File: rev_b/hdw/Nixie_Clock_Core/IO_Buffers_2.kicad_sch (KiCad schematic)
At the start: 10 parts

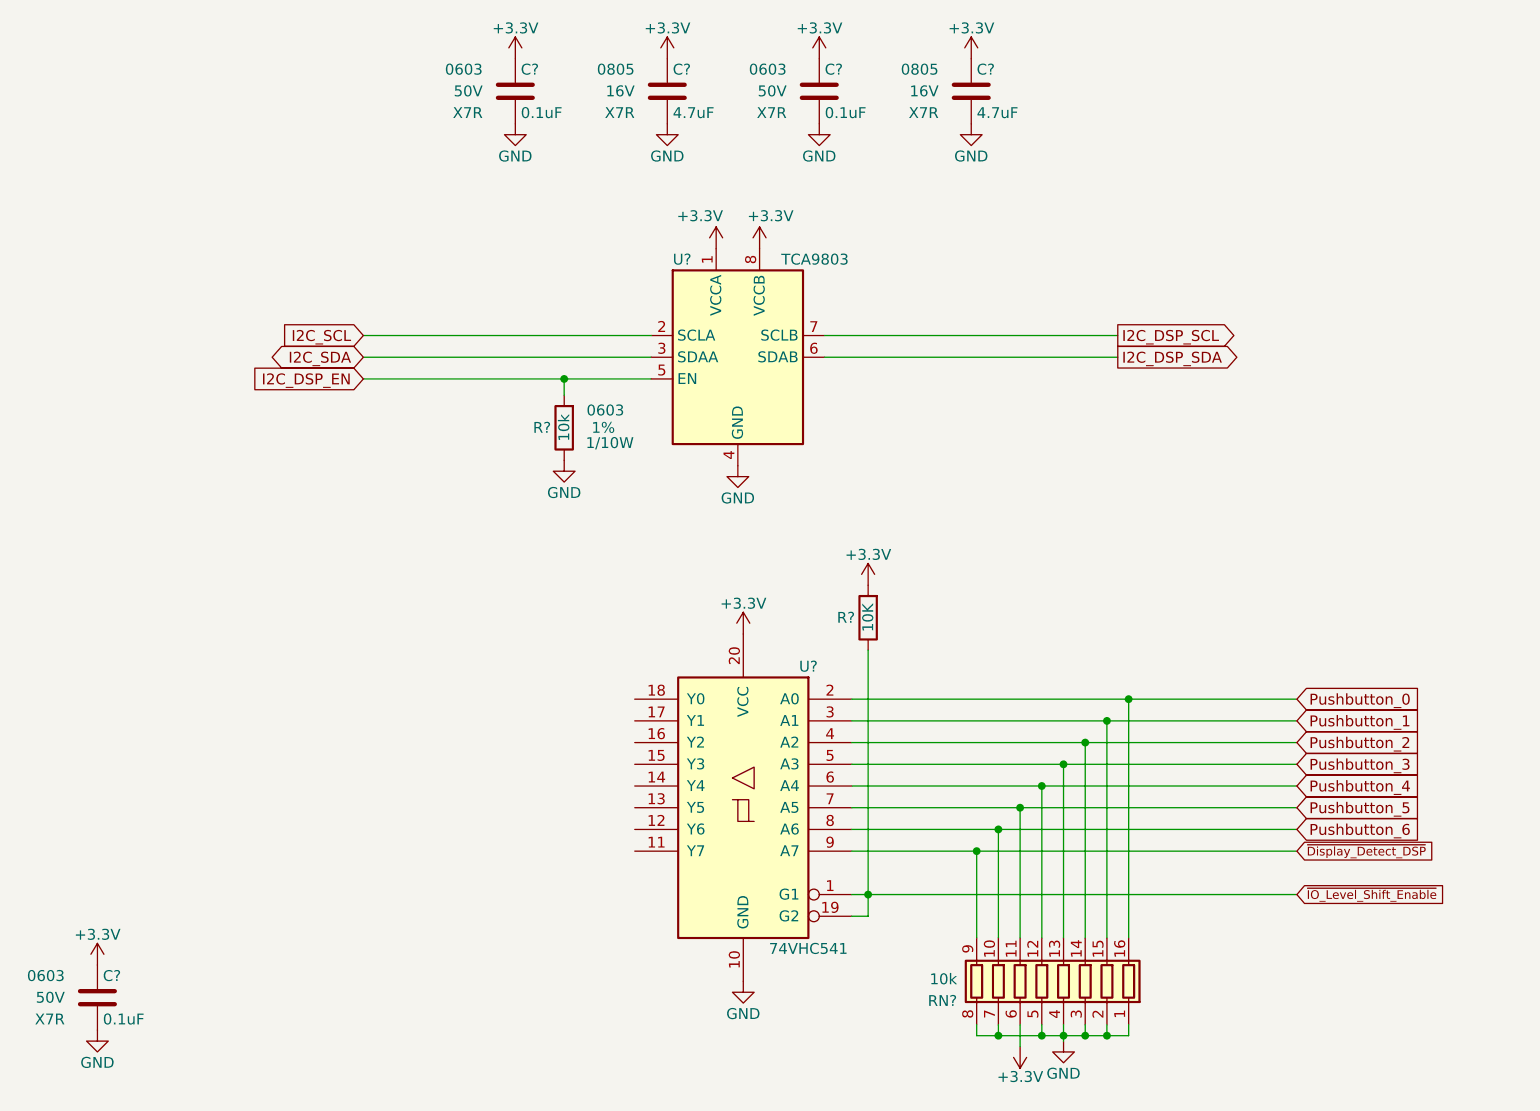
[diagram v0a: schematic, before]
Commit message: more rev b sch progress
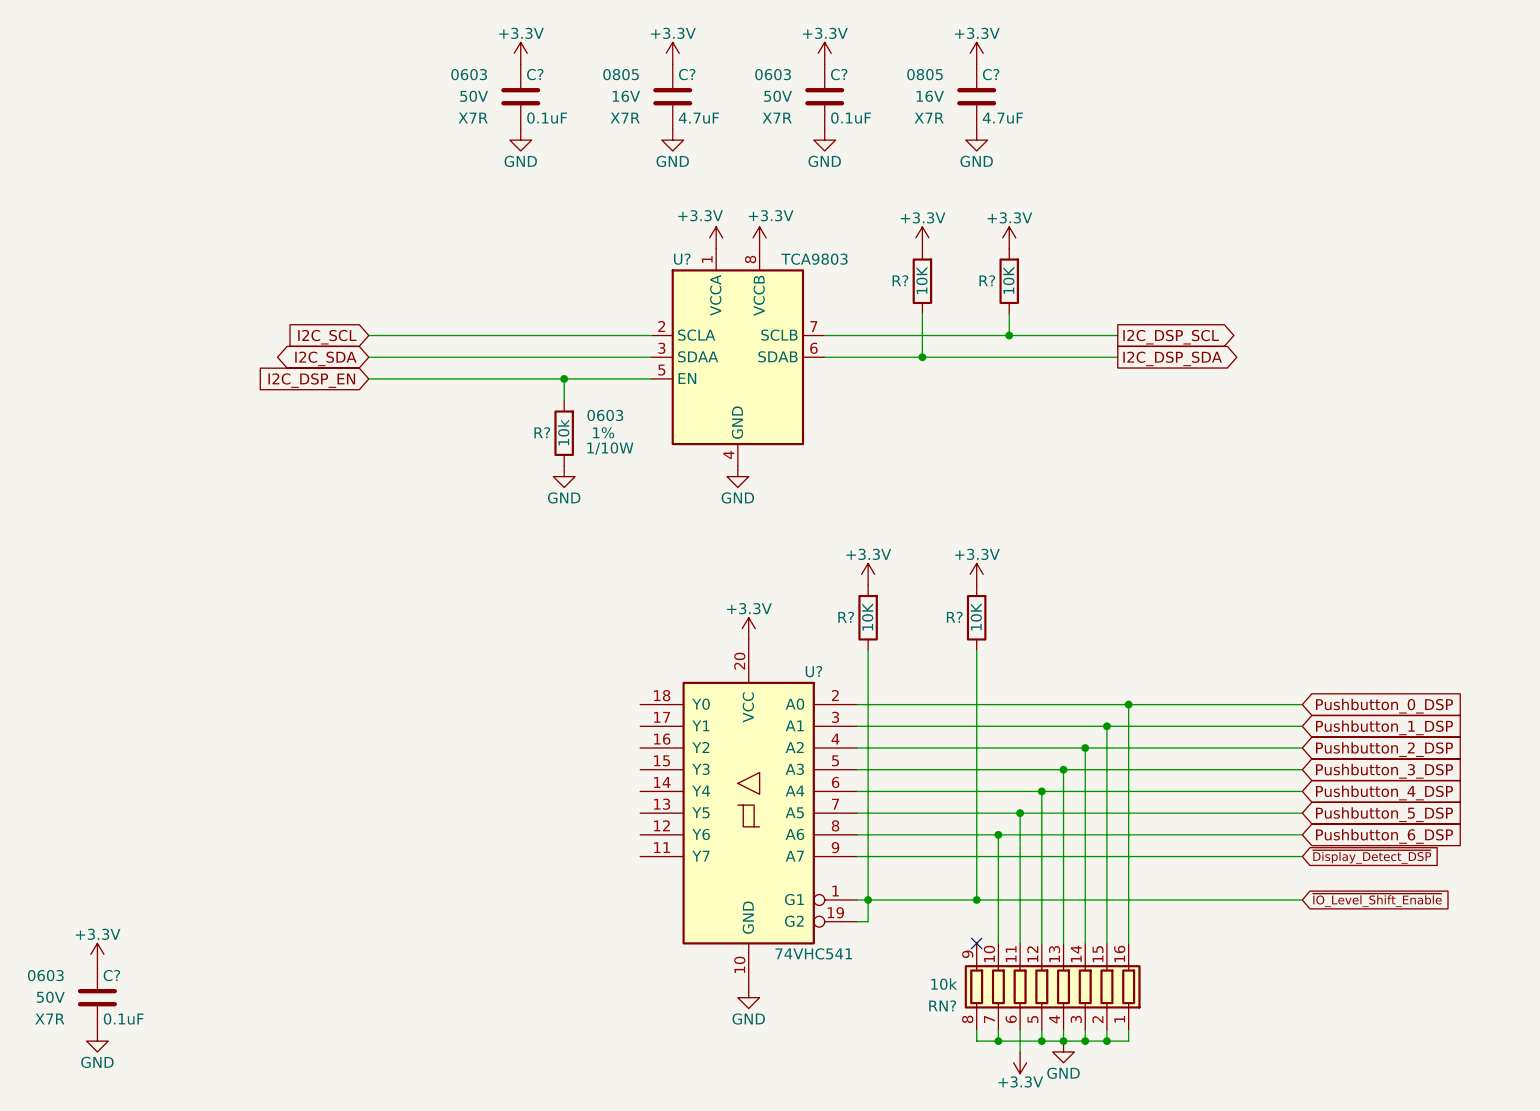
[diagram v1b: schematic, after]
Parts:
- added R? (x3): 10K, Resistors_SMD:R_0603, symbol Custom_Library:R_Custom
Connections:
- net +3.3V: now also R?.1, R?.1, R?.1
- net I2C_DSP_SCL: now also R?.2
- net I2C_DSP_SDA: now also R?.2
- net ~{Display_Detect_DSP}: no longer RN?.9 (R8.2)
- net ~{IO_Level_Shift_Enable}: now also R?.2
- net Pushbutton_0 renamed Pushbutton_0_DSP
- net Pushbutton_1 renamed Pushbutton_1_DSP
- net Pushbutton_2 renamed Pushbutton_2_DSP
- net Pushbutton_3 renamed Pushbutton_3_DSP
- net Pushbutton_4 renamed Pushbutton_4_DSP
- net Pushbutton_5 renamed Pushbutton_5_DSP
- net Pushbutton_6 renamed Pushbutton_6_DSP
- no-connect marks 0 -> 1
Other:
- moved on the sheet: C?, R?, RN?, U?

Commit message: more carrier board progress
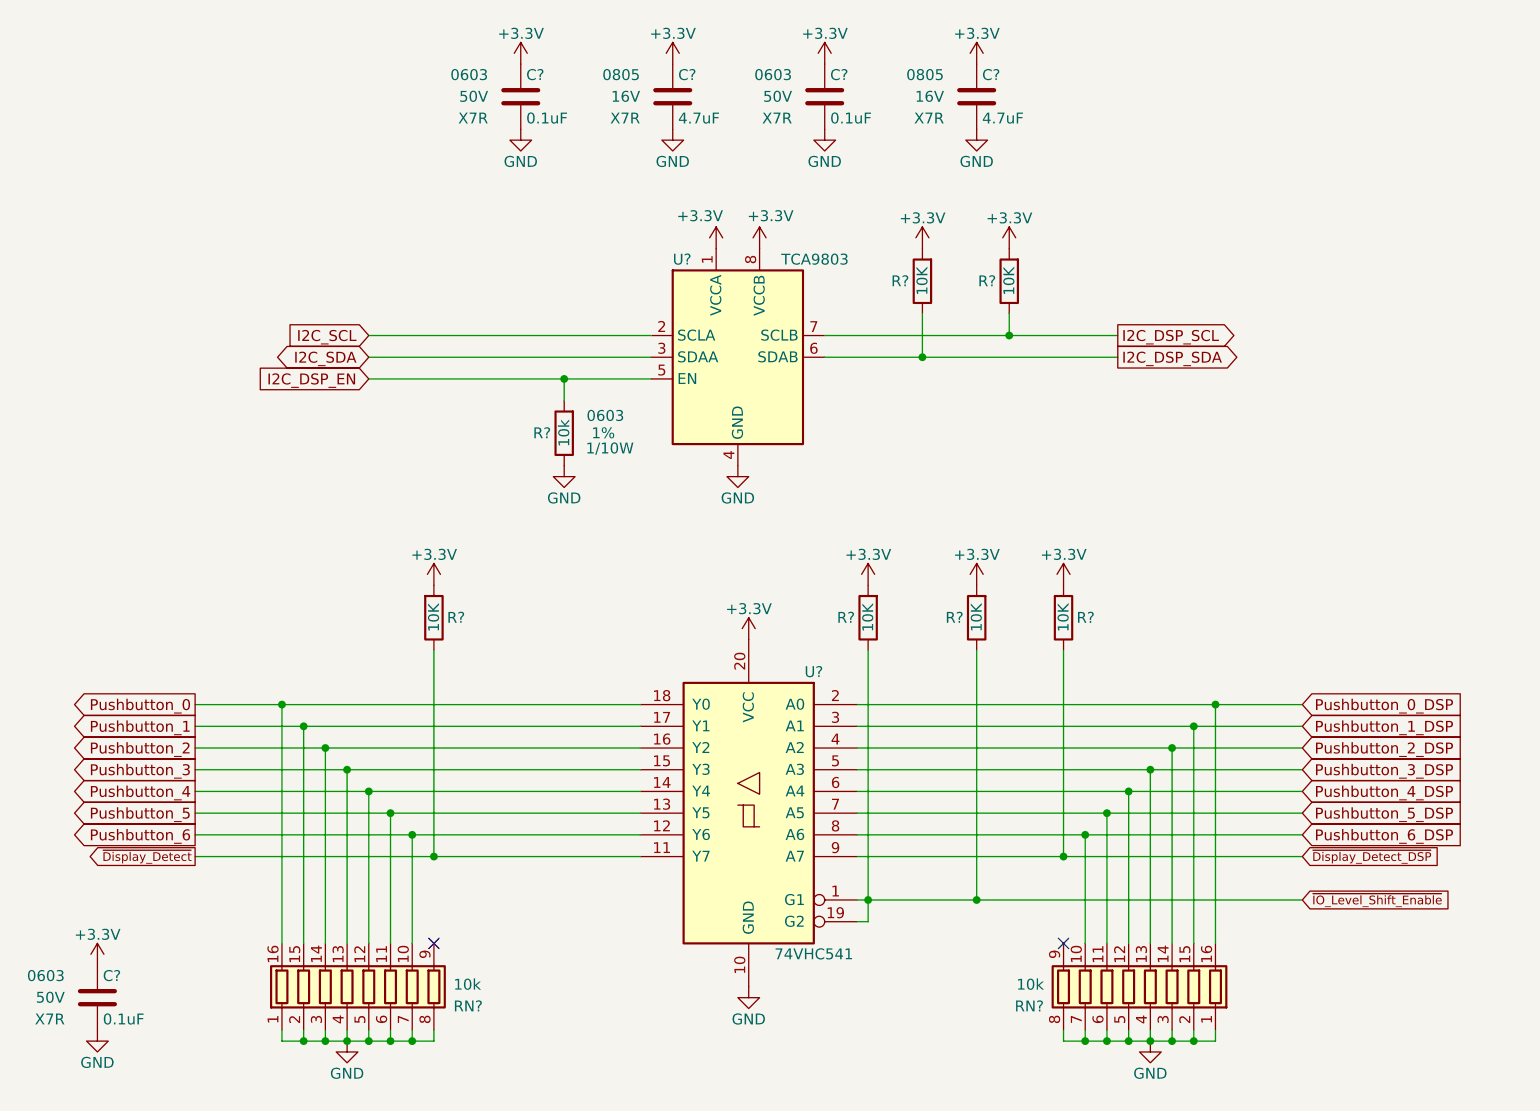
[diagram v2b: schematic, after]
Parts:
- added R? (x2): 10K, Resistors_SMD:R_0603, symbol Custom_Library:R_Custom
- added RN?: 10k, Resistors_SMD:R_Array_Convex_8x0602, symbol Device:R_Pack08
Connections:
- net +3.3V: now also R?.1, R?.1; no longer RN?.6 (R6.1)
- net GND: now also RN?.6 (R6.1), RN?.1 (R1.1), RN?.2 (R2.1), RN?.3 (R3.1), RN?.4 (R4.1), RN?.5 (R5.1), RN?.6 (R6.1), RN?.7 (R7.1), RN?.8 (R8.1)
- net ~{Display_Detect_DSP}: now also R?.2
- net ~{Display_Detect}: now reaches U?.11 (Y7)
- net ~{Display_Detect}: now also R?.2
- net Pushbutton_6: now reaches U?.12 (Y6)
- net Pushbutton_6: now also RN?.10 (R7.2)
- net Pushbutton_5: now reaches U?.13 (Y5)
- net Pushbutton_5: now also RN?.11 (R6.2)
- net Pushbutton_4: now reaches U?.14 (Y4)
- net Pushbutton_4: now also RN?.12 (R5.2)
- net Pushbutton_3: now reaches U?.15 (Y3)
- net Pushbutton_3: now also RN?.13 (R4.2)
- net Pushbutton_2: now reaches U?.16 (Y2)
- net Pushbutton_2: now also RN?.14 (R3.2)
- net Pushbutton_1: now reaches U?.17 (Y1)
- net Pushbutton_1: now also RN?.15 (R2.2)
- net Pushbutton_0: now reaches U?.18 (Y0)
- net Pushbutton_0: now also RN?.16 (R1.2)
- no-connect marks 1 -> 2
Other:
- moved on the sheet: RN?
